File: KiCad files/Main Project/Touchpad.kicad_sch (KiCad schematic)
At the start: 4 parts, among them U17 PCF8575

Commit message: update
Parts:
- R20, R21: footprint (none) -> Resistor_SMD:R_0805_2012Metric
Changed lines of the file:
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@@
       (effects (font (size 1.27 1.27)) (justify left))
     )
-    (property "Footprint" "" (id 2) (at 113.665 107.315 0)
+    (property "Footprint" "Resistor_SMD:R_0805_2012Metric" (id 2) (at 113.665 107.315 0)
       (effects (font (size 1.27 1.27)) hide)
     )
@@
       (effects (font (size 1.27 1.27)) (justify left))
     )
-    (property "Footprint" "" (id 2) (at 106.045 107.315 0)
+    (property "Footprint" "Resistor_SMD:R_0805_2012Metric" (id 2) (at 106.045 107.315 0)
       (effects (font (size 1.27 1.27)) hide)
     )

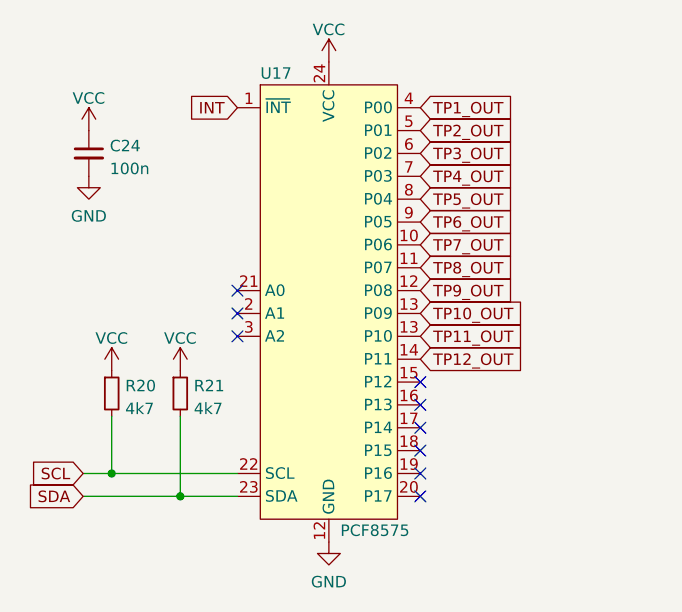
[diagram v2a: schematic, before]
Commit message: update
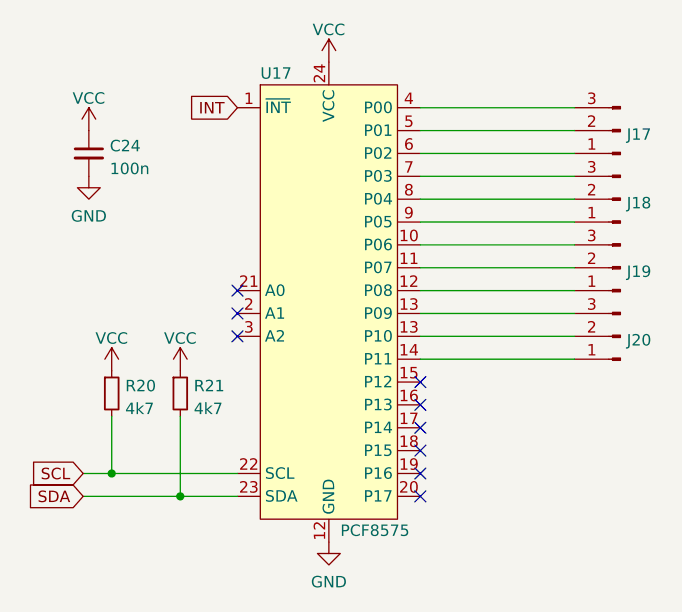
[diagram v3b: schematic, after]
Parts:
- added J17, J18, J19, J20: Conn_01x03_Male, Connector_PinHeader_2.54mm:PinHeader_1x03_P2.54mm_Vertical, symbol Connector:Conn_01x03_Male
- U17: footprint (none) -> Package_SO:SOIC-24W_7.5x15.4mm_P1.27mm
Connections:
- net TP11_OUT is gone; now on an unnamed net: U17.13 (P10)
- net TP9_OUT is gone; now on net GND: U17.12 (P08)
- net TP10_OUT: no longer names the net of U17.13 (P10)
- net TP10_OUT: now also J20.3 (Pin_3)
- net TP12_OUT: no longer names the net of U17.14 (P11)
- net TP12_OUT: now also J20.1 (Pin_1)
- net TP1_OUT: no longer names the net of U17.4 (P00)
- net TP1_OUT: now also J17.3 (Pin_3)
- net TP2_OUT: no longer names the net of U17.5 (P01)
- net TP2_OUT: now also J17.2 (Pin_2)
- net TP3_OUT: no longer names the net of U17.6 (P02)
- net TP3_OUT: now also J17.1 (Pin_1)
- net TP4_OUT: no longer names the net of U17.7 (P03)
- net TP4_OUT: now also J18.3 (Pin_3)
- net TP5_OUT: no longer names the net of U17.8 (P04)
- net TP5_OUT: now also J18.2 (Pin_2)
- net TP6_OUT: no longer names the net of U17.9 (P05)
- net TP6_OUT: now also J18.1 (Pin_1)
- net TP7_OUT: no longer names the net of U17.10 (P06)
- net TP7_OUT: now also J19.3 (Pin_3)
- net TP8_OUT: no longer names the net of U17.11 (P07)
- net TP8_OUT: now also J19.2 (Pin_2)
- new net: J19.1 (Pin_1), U17.12 (P08)
- new net: J20.2 (Pin_2), U17.13 (P10)
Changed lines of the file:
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@@
   (no_connect (at 120.015 98.425))
   (no_connect (at 120.015 95.885))
+  (wire (pts (xy 140.335 75.565) (xy 157.48 75.565))
+    (stroke (width 0) (type default) (color 0 0 0 0))
+  )
+  (wire (pts (xy 140.335 98.425) (xy 157.48 98.425))
+    (stroke (width 0) (type default) (color 0 0 0 0))
+  )
+  (wire (pts (xy 140.335 80.645) (xy 157.48 80.645))
+    (stroke (width 0) (type default) (color 0 0 0 0))
+  )
   (wire (pts (xy 113.665 109.855) (xy 113.665 118.745))
     (stroke (width 0) (type default) (color 0 0 0 0))
   )
+  (wire (pts (xy 140.335 95.885) (xy 157.48 95.885))
+    (stroke (width 0) (type default) (color 0 0 0 0))
+  )
   (wire (pts (xy 102.87 118.745) (xy 113.665 118.745))
     (stroke (width 0) (type default) (color 0 0 0 0))
   )
+  (wire (pts (xy 140.335 100.965) (xy 157.48 100.965))
+    (stroke (width 0) (type default) (color 0 0 0 0))
+  )
   (wire (pts (xy 113.665 118.745) (xy 120.015 118.745))
     (stroke (width 0) (type default) (color 0 0 0 0))
   )
+  (wire (pts (xy 140.335 83.185) (xy 157.48 83.185))
+    (stroke (width 0) (type default) (color 0 0 0 0))
+  )
   (wire (pts (xy 106.045 116.205) (xy 120.015 116.205))
     (stroke (width 0) (type default) (color 0 0 0 0))
   )
+  (wire (pts (xy 140.335 90.805) (xy 157.48 90.805))
+    (stroke (width 0) (type default) (color 0 0 0 0))
+  )
+  (wire (pts (xy 140.335 103.505) (xy 157.48 103.505))
+    (stroke (width 0) (type default) (color 0 0 0 0))
+  )
+  (wire (pts (xy 140.335 85.725) (xy 157.48 85.725))
+    (stroke (width 0) (type default) (color 0 0 0 0))
+  )
+  (wire (pts (xy 140.335 78.105) (xy 157.48 78.105))
+    (stroke (width 0) (type default) (color 0 0 0 0))
+  )
   (wire (pts (xy 102.87 116.205) (xy 106.045 116.205))
     (stroke (width 0) (type default) (color 0 0 0 0))
@@
     (stroke (width 0) (type default) (color 0 0 0 0))
   )
-  (global_label "TP10_OUT" (shape input) (at 140.335 98.425 0) (fields_autoplaced)
-    (effects (font (size 1.27 1.27)) (justify left))
-    (property "Intersheet References" "${INTERSHEET_REFS}" (id 0) (at 151.9121 98.3456 0)
-      (effects (font (size 1.27 1.27)) (justify left) hide)
-    )
-  )
-  (global_label "TP8_OUT" (shape input) (at 140.335 93.345 0) (fields_autoplaced)
-    (effects (font (size 1.27 1.27)) (justify left))
-    (property "Intersheet References" "${INTERSHEET_REFS}" (id 0) (at 150.7025 93.2656 0)
-      (effects (font (size 1.27 1.27)) (justify left) hide)
-    )
-  )
-  (global_label "TP4_OUT" (shape input) (at 140.335 83.185 0) (fields_autoplaced)
-    (effects (font (size 1.27 1.27)) (justify left))
-    (property "Intersheet References" "${INTERSHEET_REFS}" (id 0) (at 150.7025 83.1056 0)
-      (effects (font (size 1.27 1.27)) (justify left) hide)
-    )
-  )
-  (global_label "TP11_OUT" (shape input) (at 140.335 100.965 0) (fields_autoplaced)
-    (effects (font (size 1.27 1.27)) (justify left))
-    (property "Intersheet References" "${INTERSHEET_REFS}" (id 0) (at 151.9121 100.8856 0)
-      (effects (font (size 1.27 1.27)) (justify left) hide)
-    )
-  )
-  (global_label "TP6_OUT" (shape input) (at 140.335 88.265 0) (fields_autoplaced)
-    (effects (font (size 1.27 1.27)) (justify left))
-    (property "Intersheet References" "${INTERSHEET_REFS}" (id 0) (at 150.7025 88.1856 0)
-      (effects (font (size 1.27 1.27)) (justify left) hide)
-    )
-  )
-  (global_label "TP5_OUT" (shape input) (at 140.335 85.725 0) (fields_autoplaced)
-    (effects (font (size 1.27 1.27)) (justify left))
-    (property "Intersheet References" "${INTERSHEET_REFS}" (id 0) (at 150.7025 85.6456 0)
-      (effects (font (size 1.27 1.27)) (justify left) hide)
-    )
+  (wire (pts (xy 140.335 93.345) (xy 157.48 93.345))
+    (stroke (width 0) (type default) (color 0 0 0 0))
+  )
+  (wire (pts (xy 140.335 88.265) (xy 157.48 88.265))
+    (stroke (width 0) (type default) (color 0 0 0 0))
   )
   (global_label "SCL" (shape input) (at 102.87 116.205 180) (fields_autoplaced)
@@
     )
   )
-  (global_label "TP9_OUT" (shape input) (at 140.335 95.885 0) (fields_autoplaced)
-    (effects (font (size 1.27 1.27)) (justify left))
-    (property "Intersheet References" "${INTERSHEET_REFS}" (id 0) (at 150.7025 95.8056 0)
-      (effects (font (size 1.27 1.27)) (justify left) hide)
-    )
-  )
   (global_label "INT" (shape input) (at 120.015 75.565 180) (fields_autoplaced)
     (effects (font (size 1.27 1.27)) (justify right))
@@
     )
   )
-  (global_label "TP7_OUT" (shape input) (at 140.335 90.805 0) (fields_autoplaced)
-    (effects (font (size 1.27 1.27)) (justify left))
-    (property "Intersheet References" "${INTERSHEET_REFS}" (id 0) (at 150.7025 90.7256 0)
-      (effects (font (size 1.27 1.27)) (justify left) hide)
-    )
-  )
-  (global_label "TP1_OUT" (shape input) (at 140.335 75.565 0) (fields_autoplaced)
-    (effects (font (size 1.27 1.27)) (justify left))
-    (property "Intersheet References" "${INTERSHEET_REFS}" (id 0) (at 150.7025 75.4856 0)
-      (effects (font (size 1.27 1.27)) (justify left) hide)
-    )
-  )
-  (global_label "TP2_OUT" (shape input) (at 140.335 78.105 0) (fields_autoplaced)
-    (effects (font (size 1.27 1.27)) (justify left))
-    (property "Intersheet References" "${INTERSHEET_REFS}" (id 0) (at 150.7025 78.0256 0)
-      (effects (font (size 1.27 1.27)) (justify left) hide)
-    )
-  )
-  (global_label "TP12_OUT" (shape input) (at 140.335 103.505 0) (fields_autoplaced)
-    (effects (font (size 1.27 1.27)) (justify left))
-    (property "Intersheet References" "${INTERSHEET_REFS}" (id 0) (at 151.9121 103.4256 0)
-      (effects (font (size 1.27 1.27)) (justify left) hide)
-    )
-  )
-  (global_label "TP3_OUT" (shape input) (at 140.335 80.645 0) (fields_autoplaced)
-    (effects (font (size 1.27 1.27)) (justify left))
-    (property "Intersheet References" "${INTERSHEET_REFS}" (id 0) (at 150.7025 80.5656 0)
-      (effects (font (size 1.27 1.27)) (justify left) hide)
-    )
-  )
   (global_label "SDA" (shape input) (at 102.87 118.745 180) (fields_autoplaced)
     (effects (font (size 1.27 1.27)) (justify right))
@@
     )
   )
+  (symbol (lib_id "Connector:Conn_01x03_Male") (at 162.56 93.345 180) (unit 1)
+    (in_bom yes) (on_board yes) (fields_autoplaced)
+    (property "Reference" "J19" (id 0) (at 163.2712 93.7788 0)
+      (effects (font (size 1.27 1.27)) (justify right))
+    )
+    (property "Value" "Conn_01x03_Male" (id 1) (at 163.2712 95.0472 0)
+      (effects (font (size 1.27 1.27)) (justify right) hide)
+    )
+    (property "Footprint" "Connector_PinHeader_2.54mm:PinHeader_1x03_P2.54mm_Vertical" (id 2) (at 162.56 93.345 0)
+      (effects (font (size 1.27 1.27)) hide)
+    )
+    (property "Datasheet" "~" (id 3) (at 162.56 93.345 0)
+      (effects (font (size 1.27 1.27)) hide)
+    )
+    (pin "1")
+    (pin "2")
+    (pin "3")
+  )
   (symbol (lib_id "Device:C_Small") (at 103.505 80.645 0) (unit 1)
     (in_bom yes) (on_board yes) (fields_autoplaced)
@@
     )
     (pin "1")
+  )
+  (symbol (lib_id "Connector:Conn_01x03_Male") (at 162.56 100.965 180) (unit 1)
+    (in_bom yes) (on_board yes) (fields_autoplaced)
+    (property "Reference" "J20" (id 0) (at 163.2712 101.3988 0)
+      (effects (font (size 1.27 1.27)) (justify right))
+    )
+    (property "Value" "Conn_01x03_Male" (id 1) (at 163.2712 102.6672 0)
+      (effects (font (size 1.27 1.27)) (justify right) hide)
+    )
+    (property "Footprint" "Connector_PinHeader_2.54mm:PinHeader_1x03_P2.54mm_Vertical" (id 2) (at 162.56 100.965 0)
+      (effects (font (size 1.27 1.27)) hide)
+    )
+    (property "Datasheet" "~" (id 3) (at 162.56 100.965 0)
+      (effects (font (size 1.27 1.27)) hide)
+    )
+    (pin "1")
+    (pin "2")
+    (pin "3")
   )
   (symbol (lib_id "power:VCC") (at 113.665 104.775 0) (unit 1)
@@
       (effects (font (size 1.27 1.27)) (justify left))
     )
-    (property "Footprint" "" (id 2) (at 130.175 123.825 0)
+    (property "Footprint" "Package_SO:SOIC-24W_7.5x15.4mm_P1.27mm" (id 2) (at 130.175 123.825 0)
       (effects (font (size 1.27 1.27)) hide)
     )
@@
     (pin "1")
   )
+  (symbol (lib_id "Connector:Conn_01x03_Male") (at 162.56 85.725 180) (unit 1)
+    (in_bom yes) (on_board yes) (fields_autoplaced)
+    (property "Reference" "J18" (id 0) (at 163.2712 86.1588 0)
+      (effects (font (size 1.27 1.27)) (justify right))
+    )
+    (property "Value" "Conn_01x03_Male" (id 1) (at 163.2712 87.4272 0)
+      (effects (font (size 1.27 1.27)) (justify right) hide)
+    )
+    (property "Footprint" "Connector_PinHeader_2.54mm:PinHeader_1x03_P2.54mm_Vertical" (id 2) (at 162.56 85.725 0)
+      (effects (font (size 1.27 1.27)) hide)
+    )
+    (property "Datasheet" "~" (id 3) (at 162.56 85.725 0)
+      (effects (font (size 1.27 1.27)) hide)
+    )
+    (pin "1")
+    (pin "2")
+    (pin "3")
+  )
   (symbol (lib_id "power:GND") (at 103.505 83.185 0) (unit 1)
     (in_bom yes) (on_board yes) (fields_autoplaced)
@@
     (pin "1")
   )
+  (symbol (lib_id "Connector:Conn_01x03_Male") (at 162.56 78.105 180) (unit 1)
+    (in_bom yes) (on_board yes) (fields_autoplaced)
+    (property "Reference" "J17" (id 0) (at 163.2712 78.5388 0)
+      (effects (font (size 1.27 1.27)) (justify right))
+    )
+    (property "Value" "Conn_01x03_Male" (id 1) (at 163.2712 79.8072 0)
+      (effects (font (size 1.27 1.27)) (justify right) hide)
+    )
+    (property "Footprint" "Connector_PinHeader_2.54mm:PinHeader_1x03_P2.54mm_Vertical" (id 2) (at 162.56 78.105 0)
+      (effects (font (size 1.27 1.27)) hide)
+    )
+    (property "Datasheet" "~" (id 3) (at 162.56 78.105 0)
+      (effects (font (size 1.27 1.27)) hide)
+    )
+    (pin "1")
+    (pin "2")
+    (pin "3")
+  )
   (symbol (lib_id "Device:R_Small") (at 113.665 107.315 0) (unit 1)
